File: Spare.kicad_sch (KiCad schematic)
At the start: 9 parts, among them U14 74LS125, U2 74LS14, U26 74LS06, U34 74LS393, U39 74LS04, U49 74LS07N, U5 74LS02, U59 74LS32, U8 74LS08

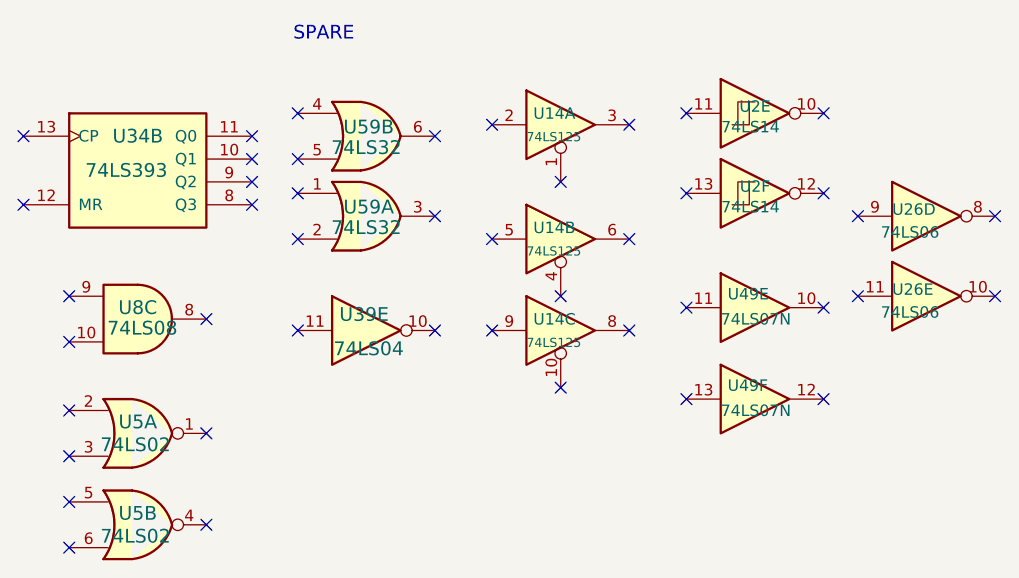
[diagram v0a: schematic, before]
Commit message: rev 1.0
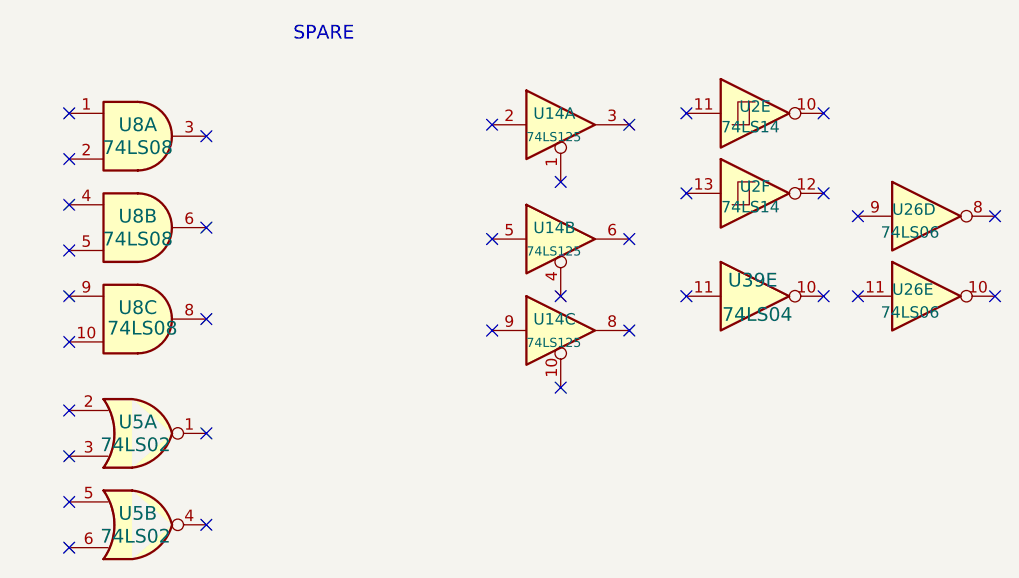
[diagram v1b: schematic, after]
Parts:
- removed U34: 74LS393, Custom:STD_DDW_DIP14, symbol 74xx:74LS393
- removed U49: 74LS07N, Custom:STD_DDW_DIP14, symbol 74xx:74LS07
- removed U59: 74LS32, Custom:STD_DDW_DIP14, symbol 74xx:74LS32
- added unit 2 of U8
- added unit 1 of U8
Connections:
- no-connect marks 44 -> 34
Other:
- moved on the sheet: U39E

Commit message: V1
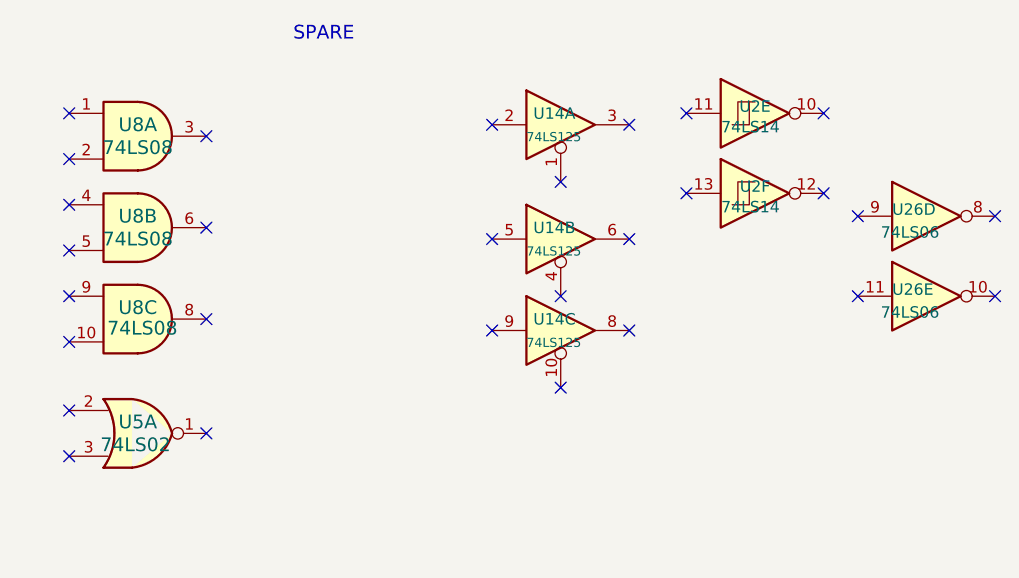
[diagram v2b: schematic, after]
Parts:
- removed U39: 74LS04, Custom:STD_DDW_DIP14, symbol 74xx:74LS04
- removed unit 2 of U5
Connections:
- no-connect marks 34 -> 29
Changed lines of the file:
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@@
-	)
-	(no_connect
-		(at 231.14 124.46)
-	)
-	(no_connect
-		(at 299.72 101.6)
 	)
 	(no_connect
@@
 	)
 	(no_connect
-		(at 231.14 129.54)
-	)
-	(no_connect
 		(at 246.38 93.98)
 	)
@@
 	)
 	(no_connect
-		(at 246.38 127)
-	)
-	(no_connect
 		(at 246.38 83.82)
 	)
@@
 	)
 	(no_connect
-		(at 314.96 101.6)
-	)
-	(no_connect
 		(at 278.13 105.41)
 	)
@@
 	(no_connect
 		(at 318.77 101.6)
-	)
-	(symbol
-		(lib_id "74xx:74LS04")
-		(at 307.34 101.6 0)
-		(unit 5)
-		(exclude_from_sim no)
-		(in_bom yes)
-		(on_board yes)
-		(dnp no)
-		(property "Reference" "U39"
-			(at 307.086 99.822 0)
-			(effects
-				(font
-					(size 1.524 1.524)
-				)
-			)
-		)
-		(property "Value" "74LS04"
-			(at 307.594 103.632 0)
-			(effects
-				(font
-					(size 1.524 1.524)
-				)
-			)
-		)
-		(property "Footprint" "Custom:STD_DDW_DIP14"
-			(at 307.34 101.6 0)
-			(effects
-				(font
-					(size 1.27 1.27)
-				)
-				(hide yes)
-			)
-		)
-		(property "Datasheet" "http://www.ti.com/lit/gpn/sn74LS04"
-			(at 307.34 101.6 0)
-			(effects
-				(font
-					(size 1.27 1.27)
-				)
-				(hide yes)
-			)
-		)
-		(property "Description" "Hex Inverter"
-			(at 307.34 101.6 0)
-			(effects
-				(font
-					(size 1.27 1.27)
-				)
-				(hide yes)
-			)
-		)
-		(pin "14"
-		)
-		(pin "7"
-		)
-		(pin "1"
-		)
-		(pin "2"
-		)
-		(pin "3"
-		)
-		(pin "4"
-		)
-		(pin "10"
-		)
-		(pin "9"
-		)
-		(pin "11"
-		)
-		(pin "8"
-		)
-		(pin "12"
-		)
-		(pin "5"
-		)
-		(pin "13"
-		)
-		(pin "6"
-		)
-		(instances
-			(project "N8PC"
-				(path "/d94f9d60-5ece-4752-b49c-b0d1c95f35bc/00000000-0000-0000-0000-0000526d48aa"
-					(reference "U39")
-					(unit 5)
-				)
-			)
-		)
 	)
 	(symbol
@@
 				)
 			)
-		)
-	)
-	(symbol
-		(lib_id "74xx:74LS02")
-		(at 238.76 127 0)
-		(unit 2)
-		(exclude_from_sim no)
-		(in_bom yes)
-		(on_board yes)
-		(dnp no)
-		(property "Reference" "U5"
-			(at 238.76 125.73 0)
-			(effects
-				(font
-					(size 1.524 1.524)
-				)
-			)
-		)
-		(property "Value" "74LS02"
-			(at 238.506 128.27 0)
-			(effects
-				(font
-					(size 1.524 1.524)
-				)
-			)
-		)
-		(property "Footprint" "Custom:STD_DDW_DIP14"
-			(at 238.76 127 0)
-			(effects
-				(font
-					(size 1.27 1.27)
-				)
-				(hide yes)
-			)
-		)
-		(property "Datasheet" "http://www.ti.com/lit/gpn/sn74ls02"
-			(at 238.76 127 0)
-			(effects
-				(font
-					(size 1.27 1.27)
-				)
-				(hide yes)
-			)
-		)
-		(property "Description" "quad 2-input NOR gate"
-			(at 238.76 127 0)
-			(effects
-				(font
-					(size 1.27 1.27)
-				)
-				(hide yes)
-			)
-		)
-		(pin "7"
-		)
-		(pin "2"
-		)
-		(pin "1"
-		)
-		(pin "14"
-		)
-		(pin "3"
-		)
-		(pin "4"
-		)
-		(pin "6"
-		)
-		(pin "10"
-		)
-		(pin "13"
-		)
-		(pin "9"
-		)
-		(pin "5"
-		)
-		(pin "12"
-		)
-		(pin "8"
-		)
-		(pin "11"
-		)
-		(instances
-			(project "N8PC"
-				(path "/d94f9d60-5ece-4752-b49c-b0d1c95f35bc/00000000-0000-0000-0000-0000526d48aa"
-					(reference "U5")
-					(unit 2)
-				)
-			)
